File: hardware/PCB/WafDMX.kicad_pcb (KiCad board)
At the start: 2 copper layers, 91.4 x 101.6 mm, 54 parts, among them J1 Wuerth_7499010121A, J2 Screw_Terminal_01x02, J3 USB_B_Micro, J4 Conn_01x04_Female, Q1 MMDT2222A, U1 AMS1117-3.3, U2 LAN8720A, U3 CH340C, U4 ESP32-WROOM-32D, U5 MAX3485, X1 ASV-50MHz

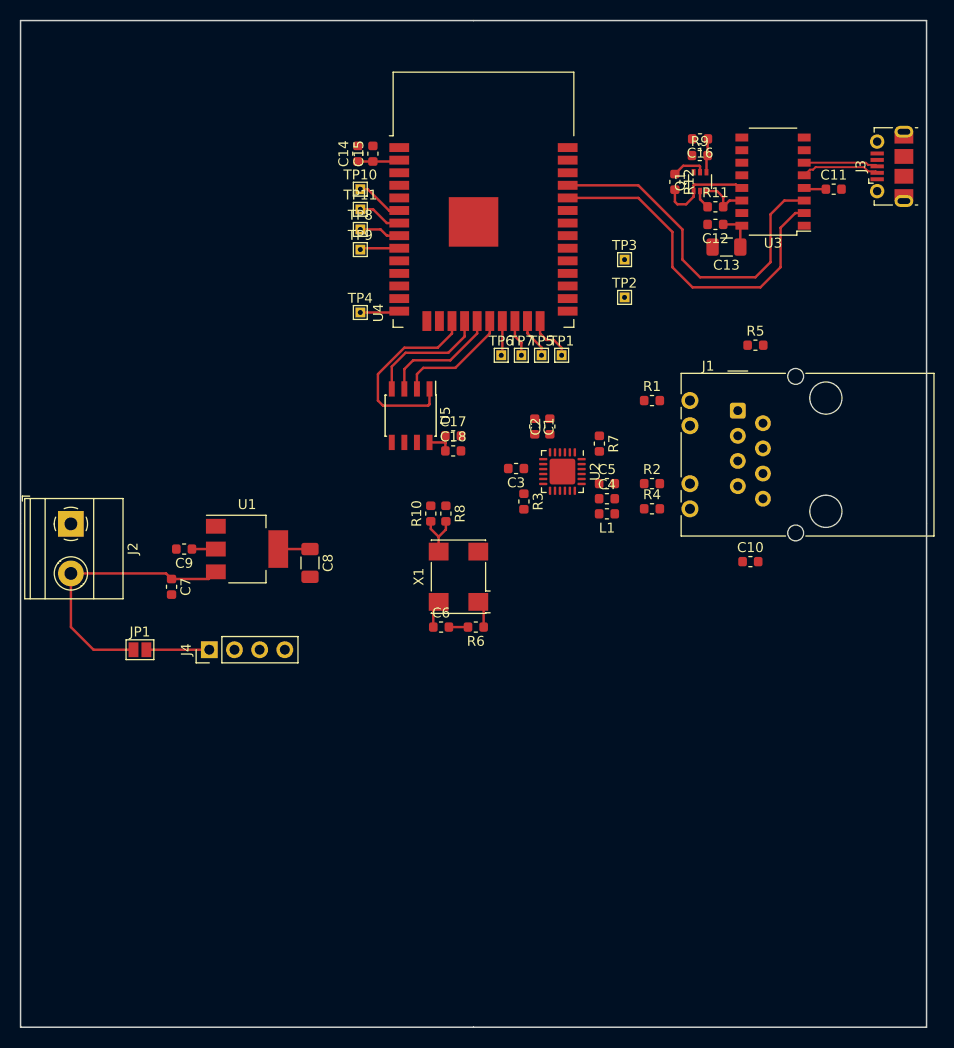
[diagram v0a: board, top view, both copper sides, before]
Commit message: Add routing
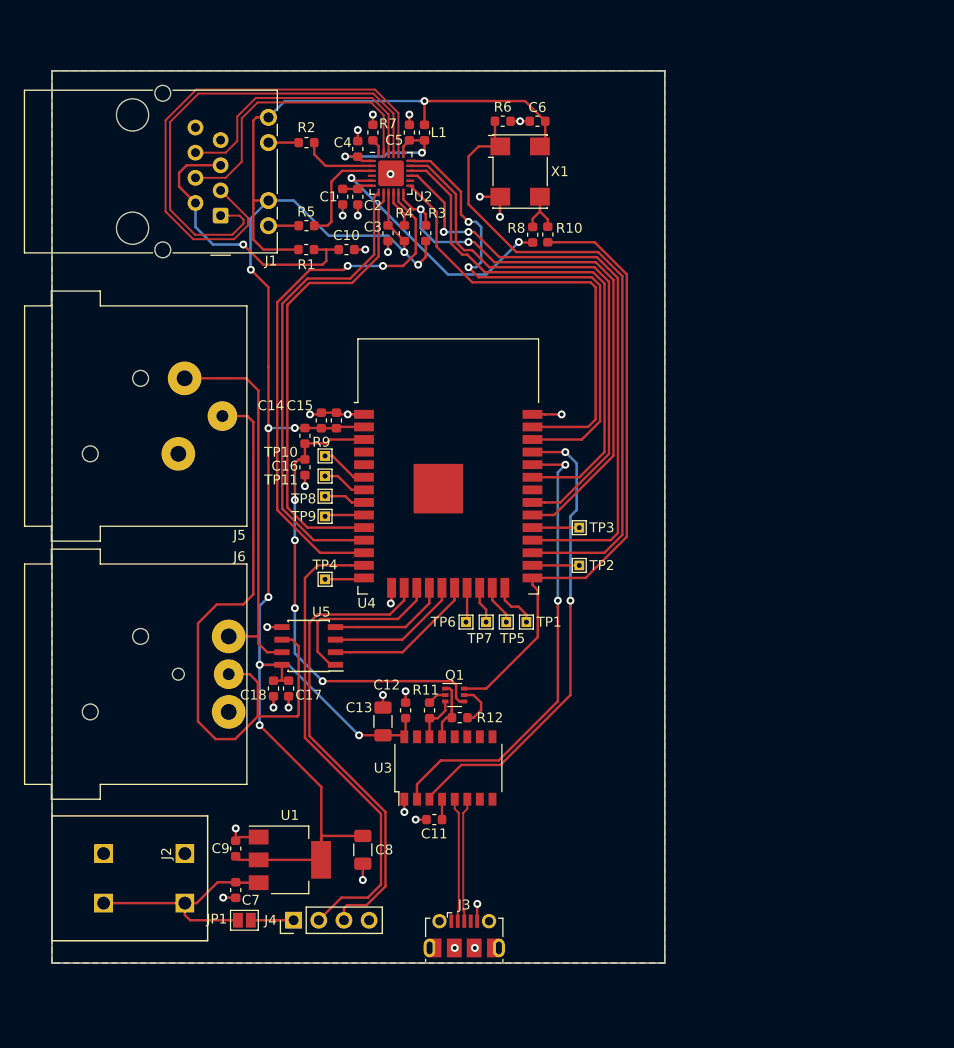
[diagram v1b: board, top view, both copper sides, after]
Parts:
- added J5: XLR3, WafDMX:XLR_Neutrik_NC3FAAH_Horizontal, F.Cu at (117.5, 94.5)
- added J6: XLR3, WafDMX:XLR_Neutrik_NC3MAAH_Horizontal, F.Cu at (117.5, 120.6)
- J2: footprint TerminalBlock_Phoenix:TerminalBlock_Phoenix_MKDS-1,5-2_1x02_P5.00mm_Horizontal -> WafDMX:TerminalBlock_WAGO_2604-1102_2x05_P5.00mm_30Degree
- R3, R4: value 33R -> 10K
- moved J3 88.8 mm to (146.4, 143.2), turned to 0 degrees
- moved C11 75.3 mm to (143.4, 131.4), turned to 180 degrees
- moved U3 67.6 mm to (144.8, 126.2), turned to 90 degrees
- moved C13 59.1 mm to (138.2, 121.5), turned to 90 degrees
- moved R11 58.4 mm to (142.9, 120.4), turned to 270 degrees
- moved R12 58.3 mm to (145.9, 121.2), turned to 180 degrees
- moved C12 58.2 mm to (140.5, 120.4), turned to 90 degrees
- moved Q1 57.4 mm to (145.4, 118.9), turned to 0 degrees
- moved J1 55.8 mm to (121.8, 70.5), turned to 180 degrees
- moved C6 52.0 mm to (153.8, 61.0), turned to 180 degrees
- moved C16 51.9 mm to (130.3, 95.9), turned to 270 degrees
- moved C10 51.5 mm to (134.5, 73.9)
- moved R6 51.1 mm to (150.3, 61.0), turned to 0 degrees
- moved R2 49.0 mm to (130.5, 63.1), turned to 180 degrees
- moved R9 48.9 mm to (130.3, 92.7), turned to 270 degrees
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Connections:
- J3 pad 1: (no net) -> Net-(J3-Pad1)
- J3 pad 4: (no net) -> Net-(J3-Pad4)
- U2 pad 14: (no net) -> Net-(U2-Pad14)
- U2 pad 4: (no net) -> Net-(U2-Pad4)
- U3 pad 10: (no net) -> Net-(U3-Pad10)
- U3 pad 11: (no net) -> Net-(U3-Pad11)
- U3 pad 12: (no net) -> Net-(U3-Pad12)
- U3 pad 15: (no net) -> Net-(U3-Pad15)
- U3 pad 7: (no net) -> Net-(U3-Pad7)
- U3 pad 8: (no net) -> Net-(U3-Pad8)
- U3 pad 9: (no net) -> Net-(U3-Pad9)
- U4 pad 32: (no net) -> Net-(U4-Pad32)
- U4 pad 4: (no net) -> Net-(U4-Pad4)
- U4 pad 5: (no net) -> Net-(U4-Pad5)
- U5 pad 6: (no net) -> Net-(J5-Pad3)
- U5 pad 7: (no net) -> Net-(J5-Pad2)
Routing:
- net +3V3: track 20.0 -> 203.3 mm, vias 0 -> 10
- net Net-(J5-Pad3): track 0.00 -> 65.0 mm
- net /PHY_CLK_EN: track 2.76 -> 65.7 mm
- net /IO0: track 0.00 -> 62.8 mm
- net /PHY_POWER: track 0.00 -> 61.6 mm, vias 0 -> 2
- net /SMI_MDIO: track 0.00 -> 56.6 mm, vias 0 -> 2
- net /EMAC_TXD0: track 0.00 -> 54.9 mm
- net /EMAC_RX_DV: track 0.00 -> 54.4 mm, vias 0 -> 2
- net /PHY_TX_N: track 0.00 -> 53.8 mm
- net /EMAC_TX_EN: track 0.00 -> 52.5 mm
- net /EMAC_TXD1: track 0.00 -> 51.6 mm, vias 0 -> 2
- net /PHY_TX_P: track 0.00 -> 49.3 mm
- net /SPI_CLK: track 0.00 -> 48.4 mm
- net /EMAC_RXD1: track 0.00 -> 48.0 mm
- net /SPI_MOSI: track 0.00 -> 47.9 mm
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- added copper zone on B.Cu, net GND
- added copper zone on F.Cu, net GND
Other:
- board size 91.4 x 101.6 mm -> 61.8 x 90 mm
